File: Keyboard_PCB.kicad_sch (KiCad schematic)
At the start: 31 parts, among them J1 USB_C_Receptacle_USB2.0_16P, J2 TC2030_SWD, U1 USBLC6-2SC6, U2 MIC5365-3.3YC5, U3 STM32F401RCT6, Y1 25MHz, Y2 32kHz768

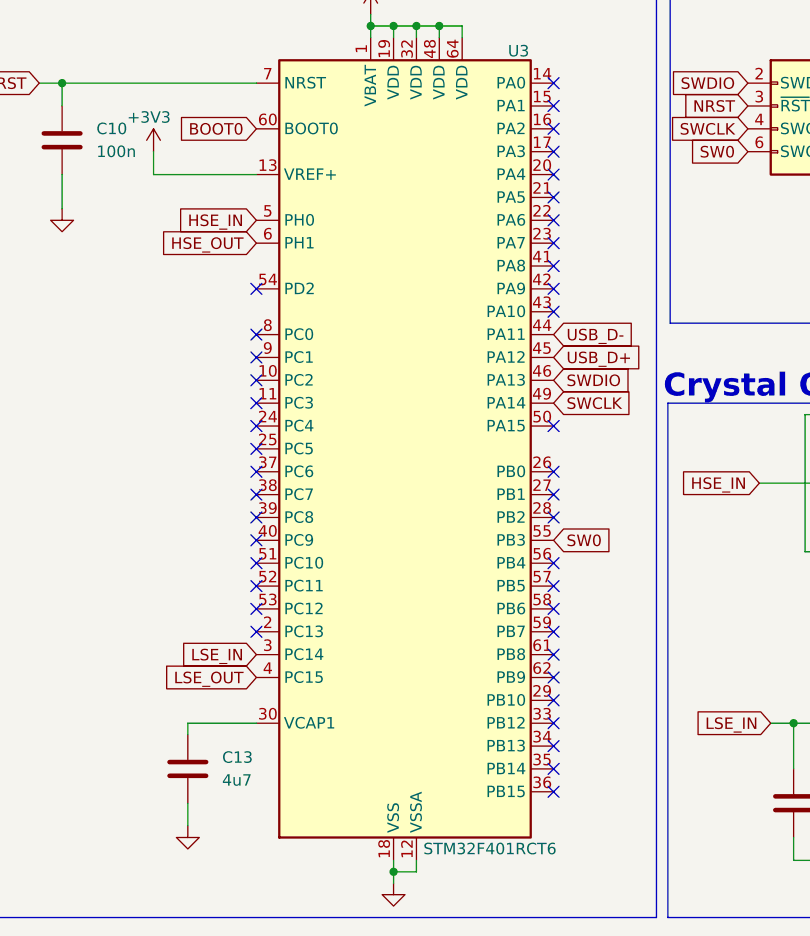
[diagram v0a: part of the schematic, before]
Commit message: PCB finished
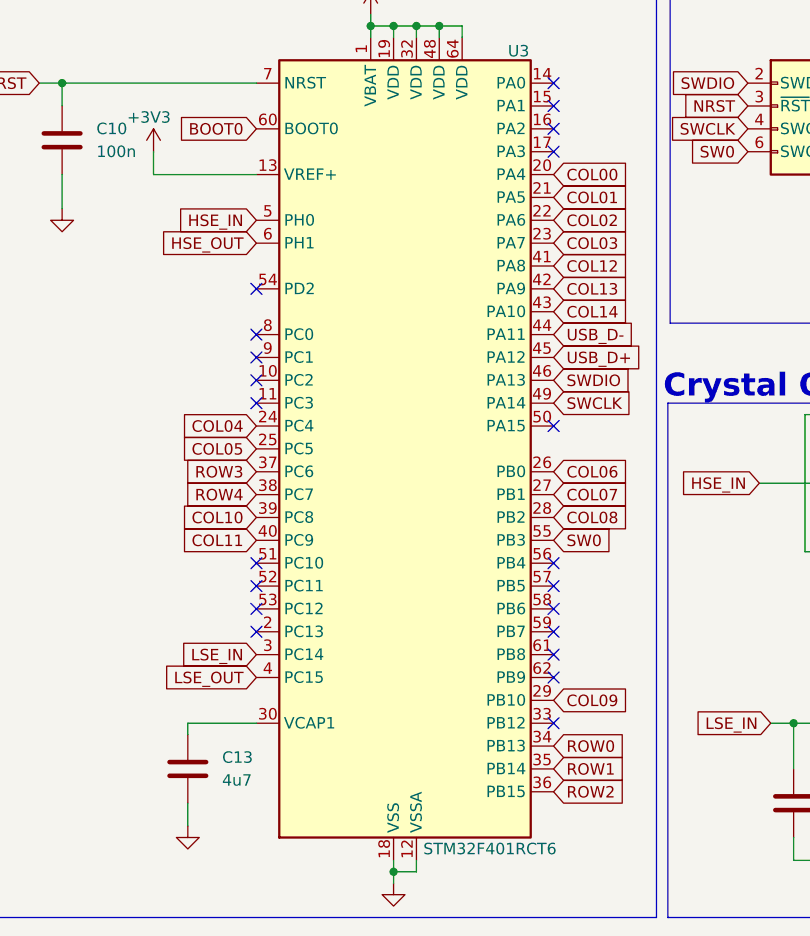
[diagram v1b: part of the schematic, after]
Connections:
- net COL00: now reaches U3.20 (PA4)
- net COL01: now reaches U3.21 (PA5)
- net COL02: now reaches U3.22 (PA6)
- net COL03: now reaches U3.23 (PA7)
- net COL04: now reaches U3.24 (PC4)
- net COL05: now reaches U3.25 (PC5)
- net COL06: now reaches U3.26 (PB0)
- net COL07: now reaches U3.27 (PB1)
- net COL08: now reaches U3.28 (PB2)
- net COL09: now reaches U3.29 (PB10)
- net ROW0: now reaches U3.34 (PB13)
- net ROW1: now reaches U3.35 (PB14)
- net ROW2: now reaches U3.36 (PB15)
- net ROW3: now reaches U3.37 (PC6)
- net ROW4: now reaches U3.38 (PC7)
- net COL10: now reaches U3.39 (PC8)
- net COL11: now reaches U3.40 (PC9)
- net COL12: now reaches U3.41 (PA8)
- net COL13: now reaches U3.42 (PA9)
- net COL14: now reaches U3.43 (PA10)
- no-connect marks 43 -> 23
